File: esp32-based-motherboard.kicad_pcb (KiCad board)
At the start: 4 copper layers, 85.4 x 83.8 mm, 122 parts, among them J1 USB_A, J10 Conn_01x02_Pin, J11 Conn_01x02_Pin, J2 USB_C_Receptacle_USB2.0_16P, J3 USB_C_Receptacle_USB2.0_16P, J4 USB_C_Receptacle_USB2.0_16P, J5 Conn_01x03_Pin, J6 Conn_01x03_Pin, J7 RJ45_Hanrun_HR911105A_Horizon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, J8 Conn_01x02_Pin, J9 Conn_01x02_Pin, SW1 SW_Push, SW2 SW_Push, SW3 SW_Push, SW4 SW_Push, SW5 SW_SPST, U1 ESP32-P4_MODULE, U2 CP2102N-Axx-xQFN24, U3 ADM3053, U4 LAN8720A, U5 LM2596S-12, U6 LM2596S-5, U7 AMS1117-3.3, Y1 25MHz

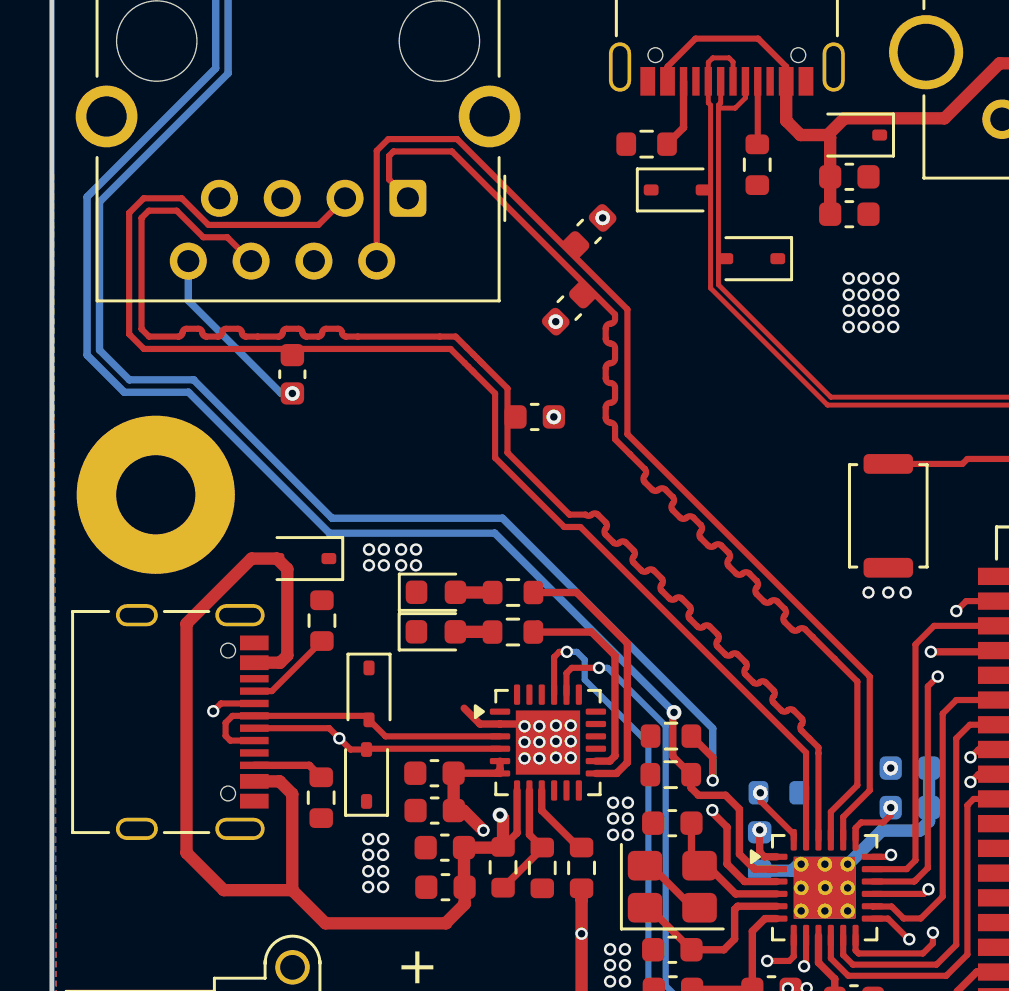
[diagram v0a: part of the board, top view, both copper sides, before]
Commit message: Updated PCB Layout
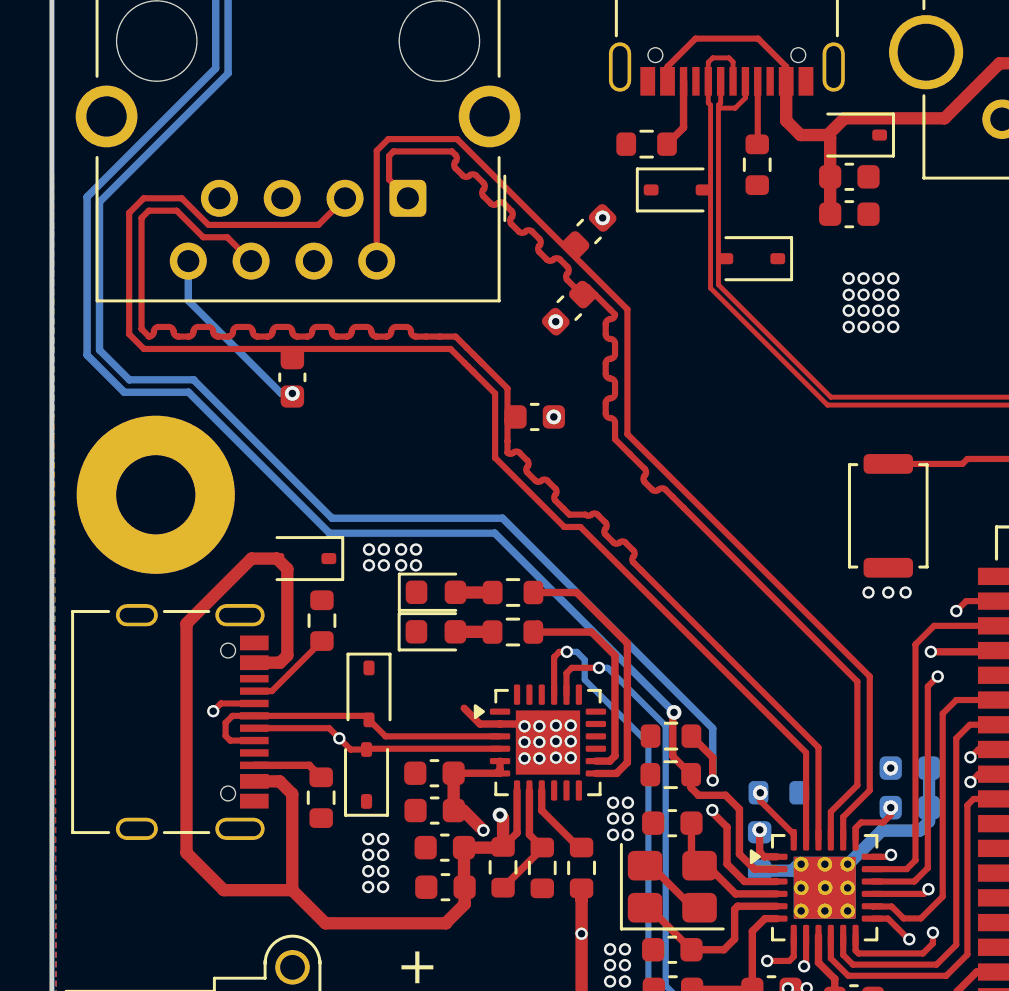
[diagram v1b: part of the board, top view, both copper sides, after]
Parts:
- moved C39 0.12 mm to (76.8, 67.1)
